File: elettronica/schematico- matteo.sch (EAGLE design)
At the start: 82 parts, among them IC1 7805T, IC2 7805T, IC3 74LS595D, J2 455-1750-1-ND, SW2 EC12E_SW

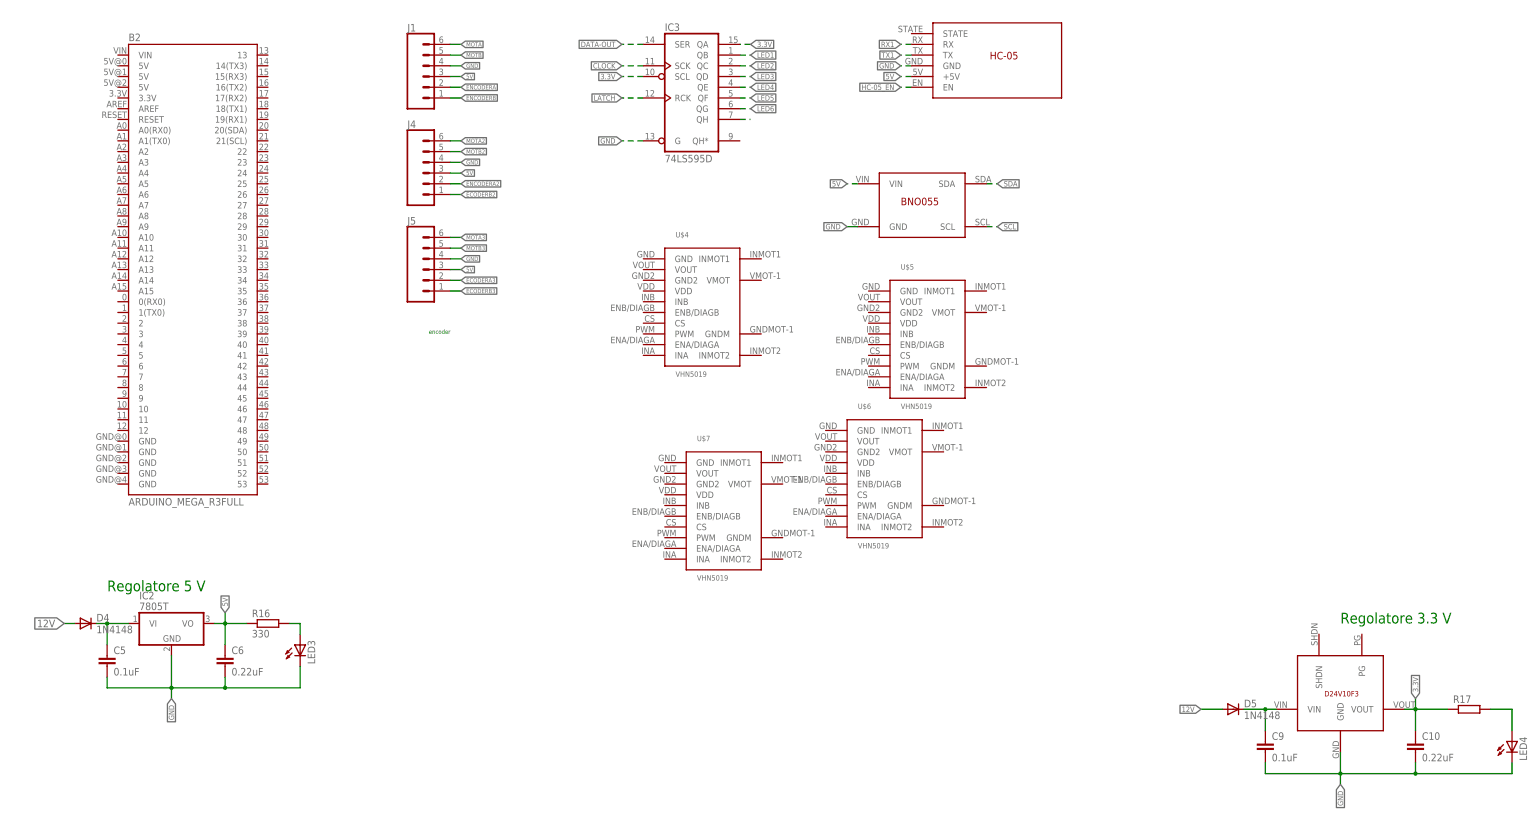
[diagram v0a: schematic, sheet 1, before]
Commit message: bla
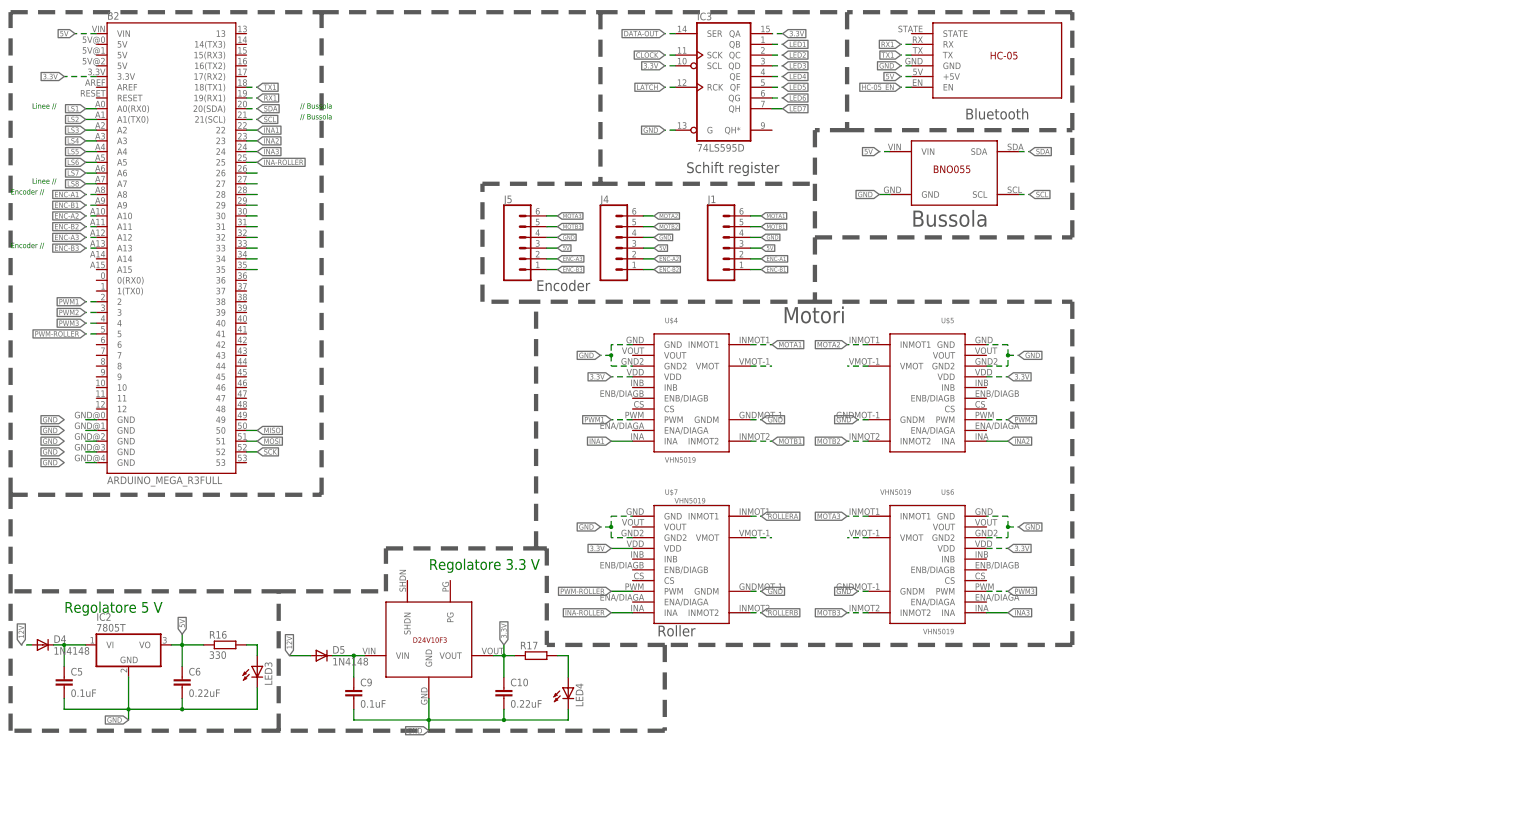
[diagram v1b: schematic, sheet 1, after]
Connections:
- removed net ECODERA3: J5.2
- removed net ECODERB2: J4.1
- removed net ECODERB3: J5.1
- removed net ENCODERA: J1.2
- removed net ENCODERA2: J4.2
- removed net ENCODERB: J1.1
- removed net MOTA: J1.6
- removed net MOTB: J1.5
- new net ENC-A1: B2.A8, J1.2
- new net ENC-A2: B2.A10, J4.2
- new net ENC-A3: B2.A12, J5.2
- new net ENC-B1: B2.A9, J1.1
- new net ENC-B2: B2.A11, J4.1
- new net ENC-B3: B2.A13, J5.1
- new net INA-ROLLER: B2.25, U$7.INA
- new net INA1: B2.22, U$4.INA
- new net INA2: B2.23, U$5.INA
- new net INA3: B2.24, U$6.INA
- new net LS1: B2.A0(RX0)
- new net LS2: B2.A1(TX0)
- new net LS3: B2.A2
- new net LS4: B2.A3
- new net LS5: B2.A4
- new net LS6: B2.A5
- new net LS7: B2.A6
- new net LS8: B2.A7
- new net MOTA1: J1.6, U$4.INMOT1
- new net MOTB1: J1.5, U$4.INMOT2
- new net N$22: B2.27
- new net N$26: B2.28
- new net N$27: B2.29
- new net N$29: B2.31
- new net N$30: B2.32
- new net N$31: B2.33
- new net N$32: B2.34
- new net N$33: B2.35
- new net N$7: B2.26
- new net PWM-ROLLER: B2.5, U$7.PWM
- new net PWM1: B2.2, U$4.PWM
- new net PWM2: B2.3, U$5.PWM
- new net PWM3: B2.4, U$6.PWM
- new net ROLLERA: U$7.INMOT1
- new net ROLLERB: U$7.INMOT2
- net 3.3V: now also B2.3.3V, U$4.VDD, U$5.VDD, U$6.VDD, U$7.VDD
- net 5V: now also B2.VIN
- net GND: now also B2.GND@0, B2.GND@1, B2.GND@2, B2.GND@3, B2.GND@4, U$4.GND, U$4.GND2, U$4.GNDM, U$5.GND, U$5.GND2, U$5.GNDM, U$6.GND, U$6.GND2, U$6.GNDM, U$7.GND, U$7.GND2, U$7.GNDM
- net LED7: now also IC3A.QH
- net MISO: now also B2.50
- net MOSI: now also B2.51
- net MOTA2: now also U$5.INMOT1
- net MOTA3: now also U$6.INMOT1
- net MOTB2: now also U$5.INMOT2
- net MOTB3: now also U$6.INMOT2
- net N$28: now also B2.30; no longer IC3A.QH
- net RX1: now also B2.19(RX1)
- net SCK: now also B2.52
- net SCL: now also B2.21(SCL)
- net SDA: now also B2.20(SDA)
- net TX1: now also B2.18(TX1)
- net VMOT: now also U$4.VMOT, U$5.VMOT, U$6.VMOT, U$7.VMOT
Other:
- note added: "// Bussola"
- note added: "Bussola"
- note added: "Encoder"
- note added: "Encoder //"
- note added: "Linee //"
- note added: "Motori"
- note added: "Roller"
- note added: "Schift register"
- note removed: "encoder"
- moved on the sheet: B2, C10, C5, C6, C9, D4, D5, IC2, IC3, J1, J4, J5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
